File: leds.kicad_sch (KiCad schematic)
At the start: 65 parts, among them U2 TXB0101DRL

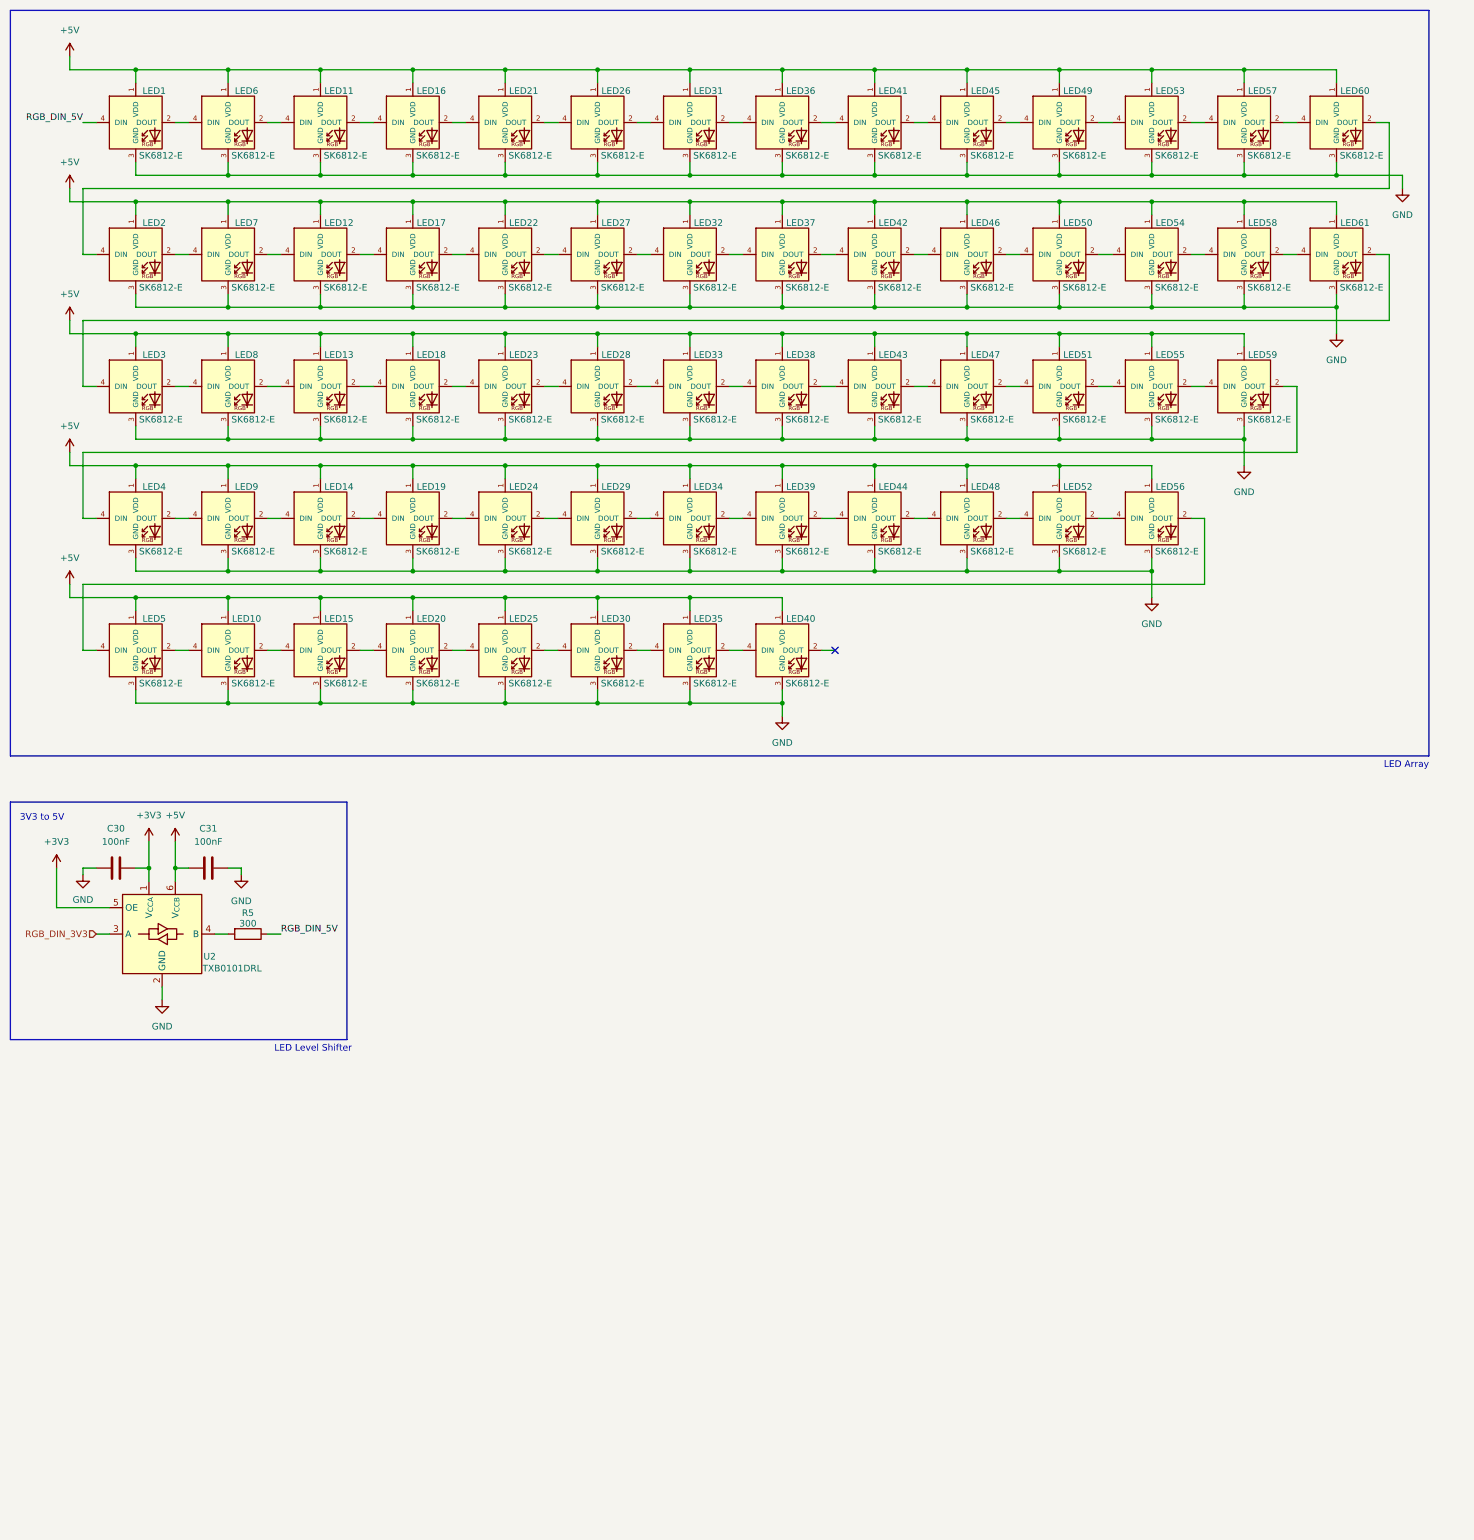
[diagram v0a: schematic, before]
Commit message: v2 done for real this time
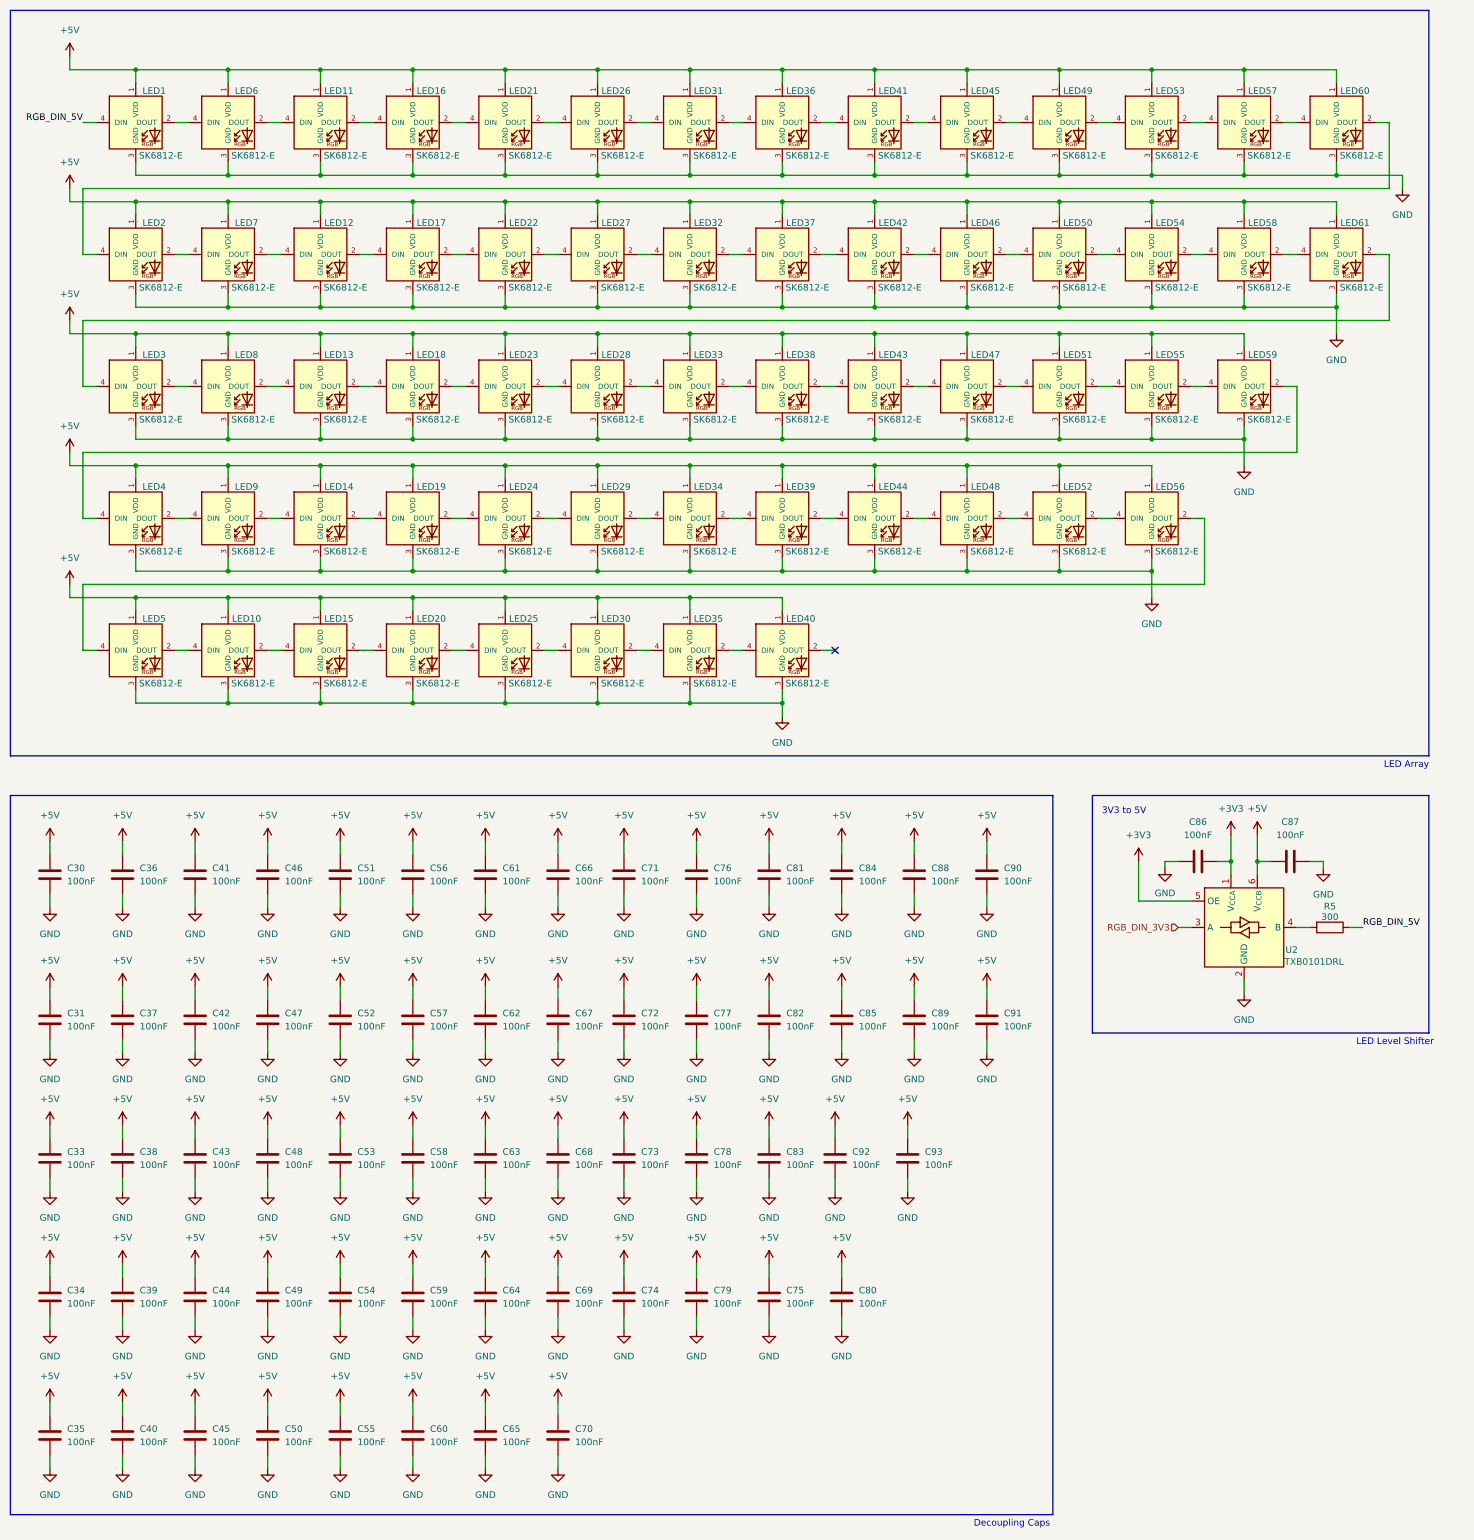
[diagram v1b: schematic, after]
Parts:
- added C30, C31, C33, C34, C35, C36, C37, C38, C39, C40, C41, C42, C43, C44, C45, C46, C47, C48, C49, C50, C51, C52, C53, C54, C55, C56, C57, C58, C59, C60, C61, C62, C63, C64, C65, C66, C67, C68, C69, C70, C71, C72, C73, C74, C75, C76, C77, C78, C79, C80, C81, C82, C83, C84, C85, C88, C89, C90, C91, C92, C93: 100nF, Capacitor_SMD:C_0402_1005Metric, symbol Device:C
- renumbered C30 to C86, C31 to C87
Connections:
- net +5V: now also C30.1, C31.1, C33.1, C34.1, C35.1, C36.1, C37.1, C38.1, C39.1, C40.1, C41.1, C42.1, C43.1, C44.1, C45.1, C46.1, C47.1, C48.1, C49.1, C50.1, C51.1, C52.1, C53.1, C54.1, C55.1, C56.1, C57.1, C58.1, C59.1, C60.1, C61.1, C62.1, C63.1, C64.1, C65.1, C66.1, C67.1, C68.1, C69.1, C70.1, C71.1, C72.1, C73.1, C74.1, C75.1, C76.1, C77.1, C78.1, C79.1, C80.1, C81.1, C82.1, C83.1, C84.1, C85.1, C88.1, C89.1, C90.1, C91.1, C92.1, C93.1
- net GND: now also C30.2, C31.2, C33.2, C34.2, C35.2, C36.2, C37.2, C38.2, C39.2, C40.2, C41.2, C42.2, C43.2, C44.2, C45.2, C46.2, C47.2, C48.2, C49.2, C50.2, C51.2, C52.2, C53.2, C54.2, C55.2, C56.2, C57.2, C58.2, C59.2, C60.2, C61.2, C62.2, C63.2, C64.2, C65.2, C66.2, C67.2, C68.2, C69.2, C70.2, C71.2, C72.2, C73.2, C74.2, C75.2, C76.2, C77.2, C78.2, C79.2, C80.2, C81.2, C82.2, C83.2, C84.2, C85.2, C88.2, C89.2, C90.2, C91.2, C92.2, C93.2
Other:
- note added: "Decoupling Caps"
- moved on the sheet: C86, C87, R5, U2
